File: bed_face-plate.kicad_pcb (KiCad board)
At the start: 2 copper layers, 228.6 x 76.2 mm, 52 parts

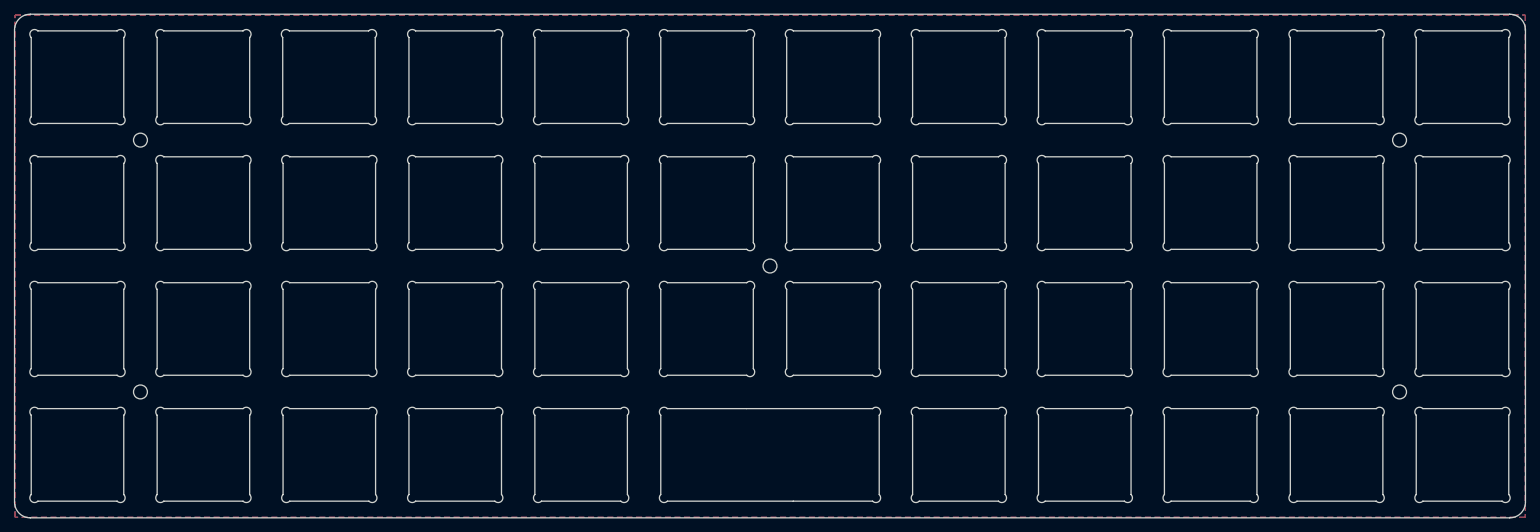
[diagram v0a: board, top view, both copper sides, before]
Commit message: initial plate from keebio dxf
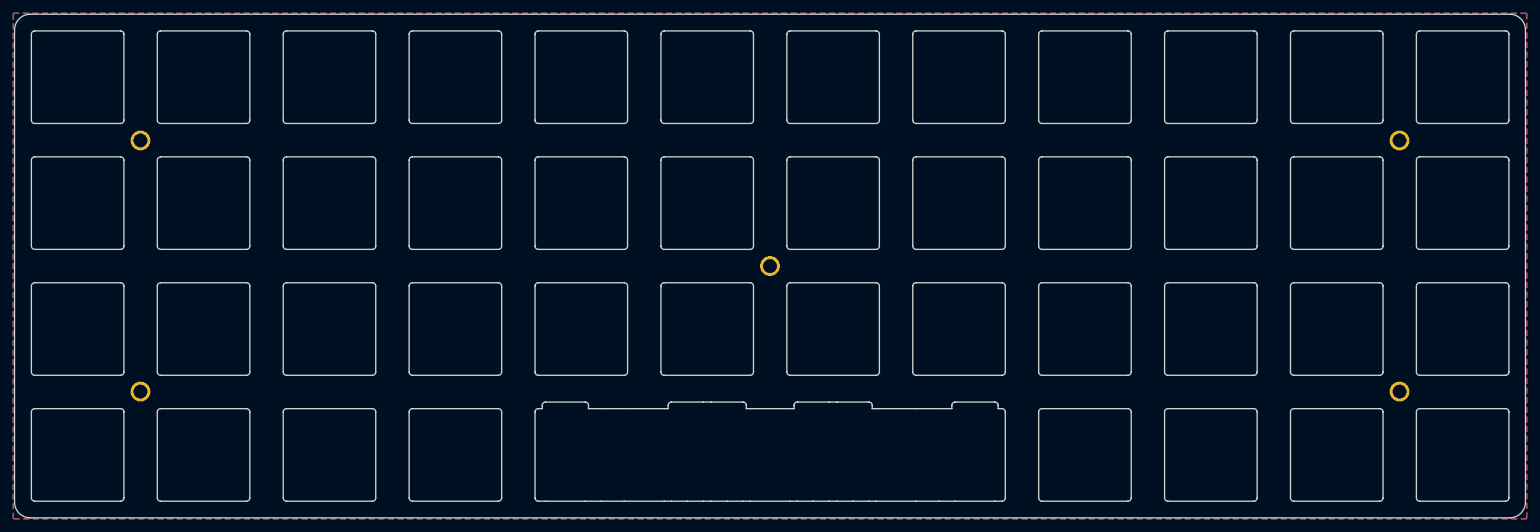
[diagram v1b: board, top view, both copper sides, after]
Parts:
- removed MX1: ESC, bed-face-components:MX-1U-PlateCutout-EDIT
- removed MX10: O, bed-face-components:MX-1U-PlateCutout-EDIT
- removed MX11: P, bed-face-components:MX-1U-PlateCutout-EDIT
- removed MX12: BACKSPACE, bed-face-components:MX-1U-PlateCutout-EDIT
- removed MX13: TAB, bed-face-components:MX-1U-PlateCutout-EDIT
- removed MX14: A, bed-face-components:MX-1U-PlateCutout-EDIT
- removed MX15: S, bed-face-components:MX-1U-PlateCutout-EDIT
- removed MX16: D, bed-face-components:MX-1U-PlateCutout-EDIT
- removed MX17: F, bed-face-components:MX-1U-PlateCutout-EDIT
- removed MX18: G, bed-face-components:MX-1U-PlateCutout-EDIT
- removed MX19: H, bed-face-components:MX-1U-PlateCutout-EDIT
- removed MX2: Q, bed-face-components:MX-1U-PlateCutout-EDIT
- removed MX20: J, bed-face-components:MX-1U-PlateCutout-EDIT
- removed MX21: K, bed-face-components:MX-1U-PlateCutout-EDIT
- removed MX22: L, bed-face-components:MX-1U-PlateCutout-EDIT
- removed MX23: ; :, bed-face-components:MX-1U-PlateCutout-EDIT
- removed MX24: ' ", bed-face-components:MX-1U-PlateCutout-EDIT
- removed MX25: SHIFT, bed-face-components:MX-1U-PlateCutout-EDIT
- removed MX26: Z, bed-face-components:MX-1U-PlateCutout-EDIT
- removed MX27: X, bed-face-components:MX-1U-PlateCutout-EDIT
- removed MX28: C, bed-face-components:MX-1U-PlateCutout-EDIT
- removed MX29: V, bed-face-components:MX-1U-PlateCutout-EDIT
- removed MX3: W, bed-face-components:MX-1U-PlateCutout-EDIT
- removed MX30: B, bed-face-components:MX-1U-PlateCutout-EDIT
- removed MX31: N, bed-face-components:MX-1U-PlateCutout-EDIT
- removed MX32: M, bed-face-components:MX-1U-PlateCutout-EDIT
- removed MX33: , <, bed-face-components:MX-1U-PlateCutout-EDIT
- removed MX34: . >, bed-face-components:MX-1U-PlateCutout-EDIT
- removed MX35: / ?, bed-face-components:MX-1U-PlateCutout-EDIT
- removed MX36: ENTER, bed-face-components:MX-1U-PlateCutout-EDIT
- removed MX37: CTRL, bed-face-components:MX-1U-PlateCutout-EDIT
- removed MX38: GUI, bed-face-components:MX-1U-PlateCutout-EDIT
- removed MX39: ALT, bed-face-components:MX-1U-PlateCutout-EDIT
- removed MX4: E, bed-face-components:MX-1U-PlateCutout-EDIT
- removed MX40: FN, bed-face-components:MX-1U-PlateCutout-EDIT
- removed MX41: LOWER, bed-face-components:MX-1U-PlateCutout-EDIT
- removed MX42: SPACE, bed-face-components:MX-2U-PlateCutout-EDIT
- removed MX44: RAISE, bed-face-components:MX-1U-PlateCutout-EDIT
- removed MX45: LEFT, bed-face-components:MX-1U-PlateCutout-EDIT
- removed MX46: DOWN, bed-face-components:MX-1U-PlateCutout-EDIT
- removed MX47: UP, bed-face-components:MX-1U-PlateCutout-EDIT
- removed MX48: RIGHT, bed-face-components:MX-1U-PlateCutout-EDIT
- removed MX5: R, bed-face-components:MX-1U-PlateCutout-EDIT
- removed MX6: T, bed-face-components:MX-1U-PlateCutout-EDIT
- removed MX7: Y, bed-face-components:MX-1U-PlateCutout-EDIT
- removed MX8: U, bed-face-components:MX-1U-PlateCutout-EDIT
- removed MX9: I, bed-face-components:MX-1U-PlateCutout-EDIT
- added P1: plate, bed-face-components:plate, F.Cu at (149.2, 104.0)
- H1, H2, H3, H4, H5: value Hole -> MountingHole_Pad; footprint bed-face-components:screw_hole -> bed-face-components:2.1mm_Screw_Hole
- moved H5 217.6 mm to (40.0, 48.7)
- moved H4 38.0 mm to (244.5, 123.0)
